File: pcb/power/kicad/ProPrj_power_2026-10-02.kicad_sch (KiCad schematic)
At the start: 0 parts

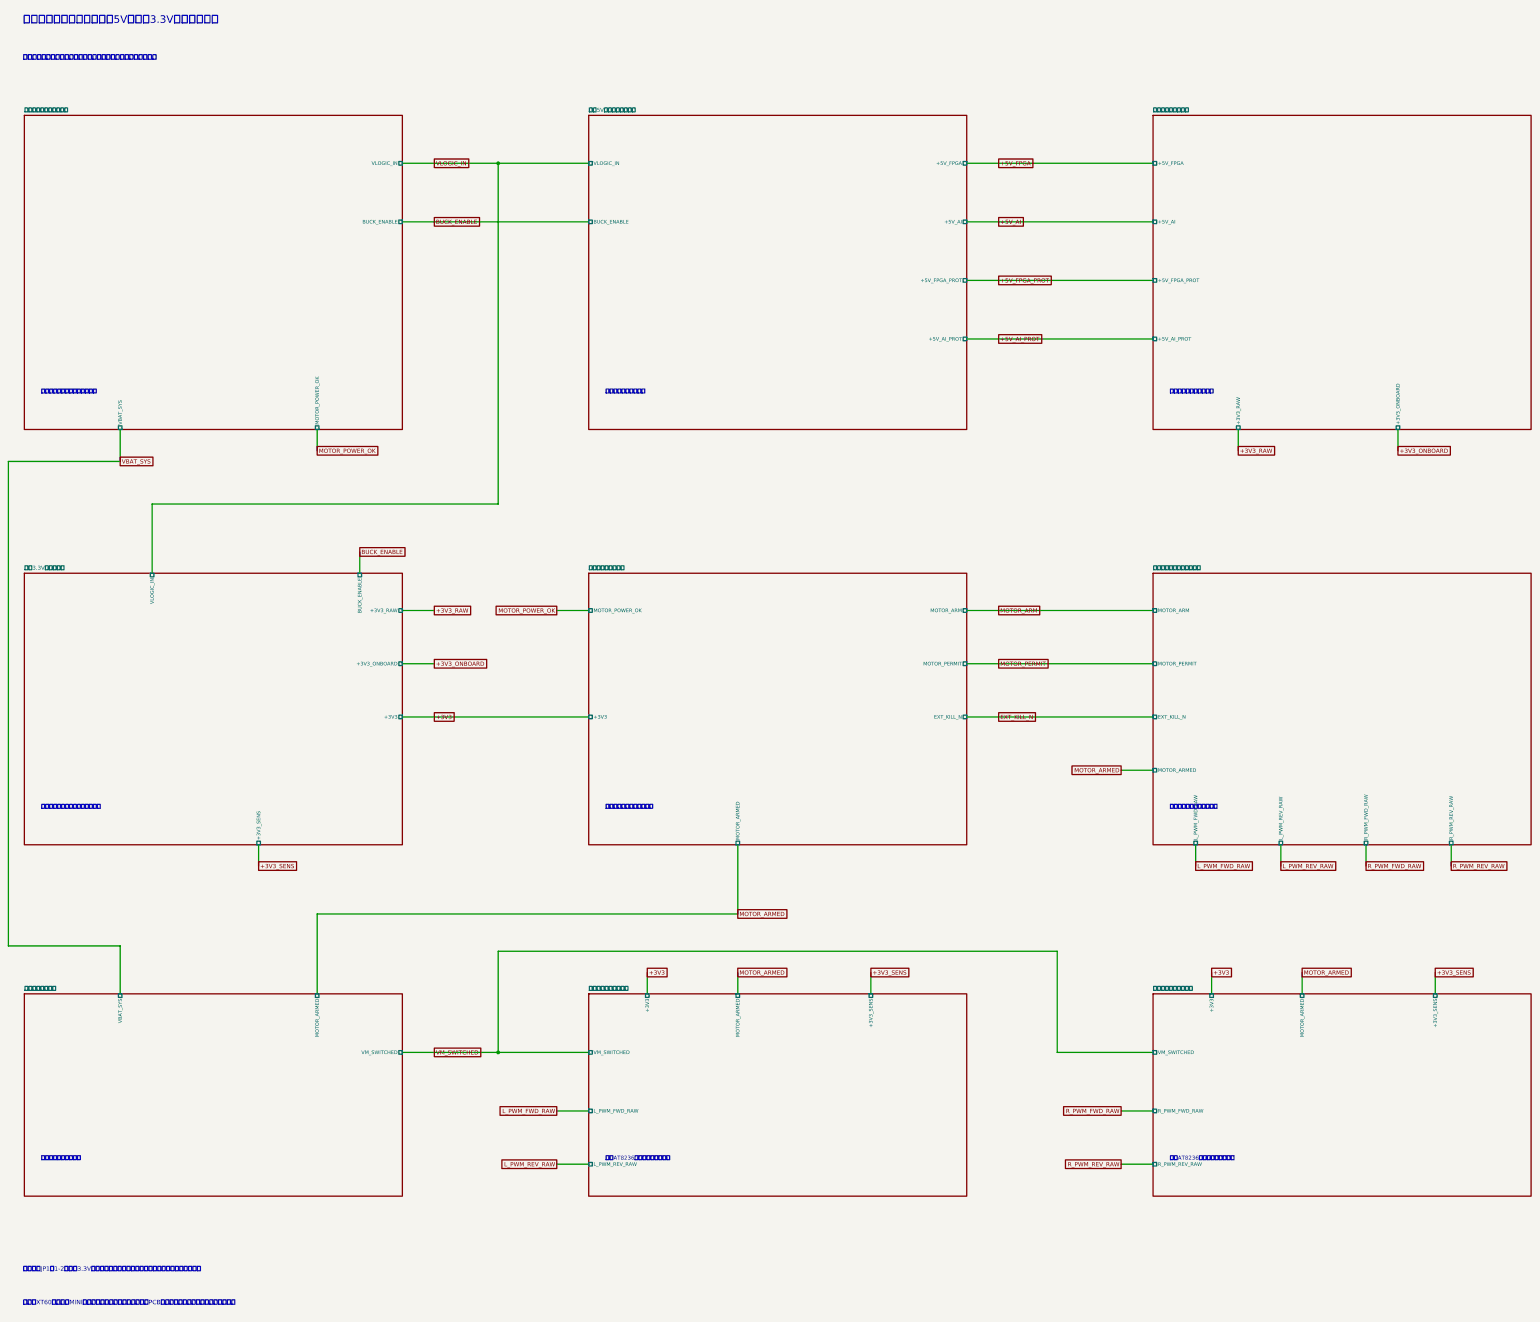
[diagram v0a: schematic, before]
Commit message: 10.4
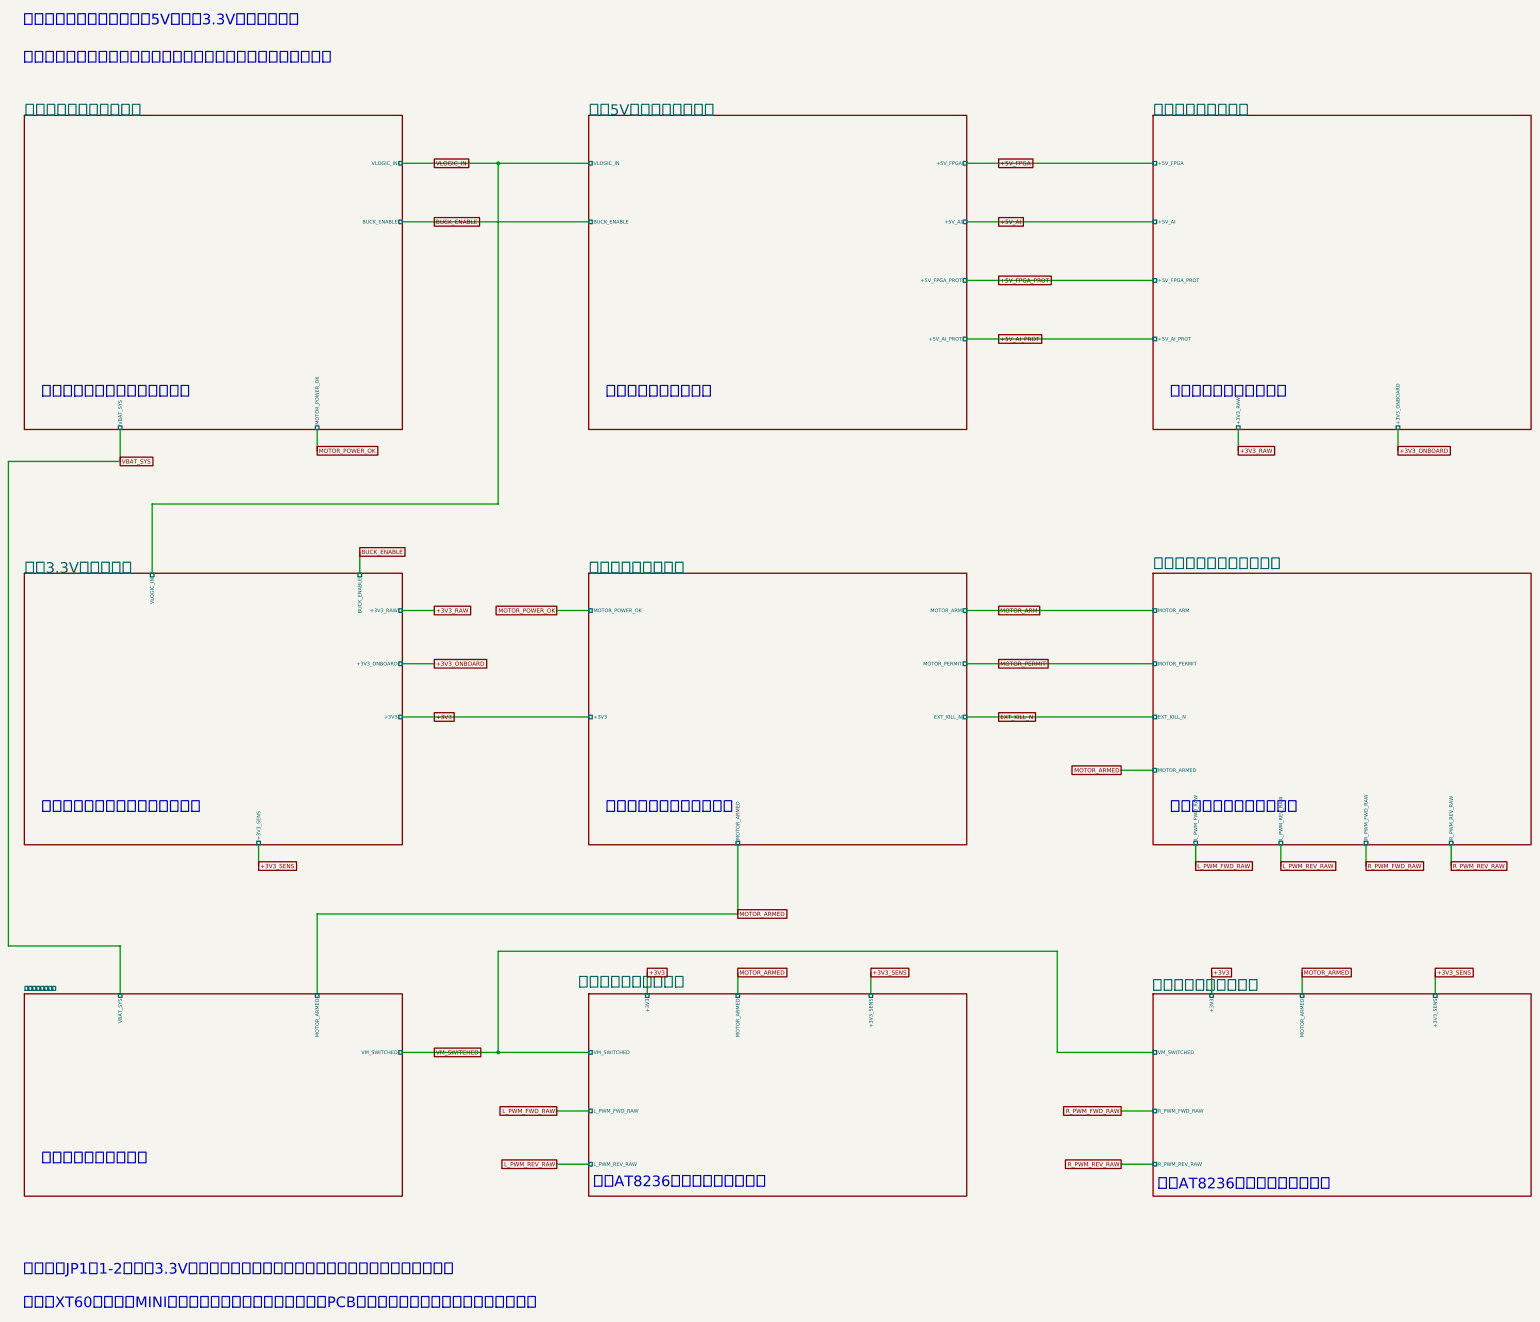
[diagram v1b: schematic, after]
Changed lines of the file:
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@@
 		(effects
 			(font
-				(size 0.95 0.95)
+				(size 2.54 2.54)
 			)
 			(justify left)
@@
 		(effects
 			(font
-				(size 1.05 1.05)
+				(size 2.54 2.54)
 			)
 			(justify left)
@@
 	(text "右侧AT8236、编码器与电流监测"
 		(exclude_from_sim no)
-		(at 293.56 289.56 0)
-		(effects
-			(font
-				(size 0.95 0.95)
+		(at 290.576 295.656 0)
+		(effects
+			(font
+				(size 2.54 2.54)
 			)
 			(justify left)
@@
 		(effects
 			(font
-				(size 0.95 0.95)
+				(size 2.54 2.54)
 			)
 			(justify left)
@@
 		(effects
 			(font
-				(size 0.95 0.95)
+				(size 2.54 2.54)
 			)
 			(justify left)
@@
 		(effects
 			(font
-				(size 0.95 0.95)
+				(size 2.54 2.54)
 			)
 			(justify left)
@@
 		(effects
 			(font
-				(size 1.1 1.1)
+				(size 2.54 2.54)
 			)
 			(justify left)
@@
 		(effects
 			(font
-				(size 0.95 0.95)
+				(size 2.54 2.54)
 			)
 			(justify left)
@@
 	(text "左侧AT8236、编码器与电流监测"
 		(exclude_from_sim no)
-		(at 158.94 289.56 0)
-		(effects
-			(font
-				(size 0.95 0.95)
+		(at 155.956 295.148 0)
+		(effects
+			(font
+				(size 2.54 2.54)
 			)
 			(justify left)
@@
 		(effects
 			(font
-				(size 0.95 0.95)
+				(size 2.54 2.54)
 			)
 			(justify left)
@@
 		(effects
 			(font
-				(size 0.95 0.95)
+				(size 2.54 2.54)
 			)
 			(justify left)
@@
 		(effects
 			(font
-				(size 1.05 1.05)
+				(size 2.54 2.54)
 			)
 			(justify left)
@@
 		(effects
 			(font
-				(size 1.8 1.8)
+				(size 2.54 2.54)
 			)
 			(justify left)
@@
 		)
 		(property "Sheetname" "右电机驱动与电流监测"
-			(at 289.56 248.92 0)
-			(show_name no)
-			(do_not_autoplace no)
-			(effects
-				(font
-					(size 0.95 0.95)
+			(at 289.306 248.158 0)
+			(show_name no)
+			(do_not_autoplace no)
+			(effects
+				(font
+					(size 2.54 2.54)
 				)
 				(justify left)
@@
 					(size 0.85 0.85)
 				)
+				(justify left)
 			)
 		)
@@
 					(size 0.85 0.85)
 				)
+				(justify right)
 			)
 		)
@@
 					(size 0.85 0.85)
 				)
+				(justify right)
 			)
 		)
@@
 					(size 0.85 0.85)
 				)
+				(justify right)
 			)
 		)
@@
 					(size 0.85 0.85)
 				)
+				(justify left)
 			)
 		)
@@
 					(size 0.85 0.85)
 				)
+				(justify left)
 			)
 		)
@@
 		)
 		(property "Sheetname" "左电机驱动与电流监测"
-			(at 154.94 248.92 0)
-			(show_name no)
-			(do_not_autoplace no)
-			(effects
-				(font
-					(size 0.95 0.95)
+			(at 152.4 247.396 0)
+			(show_name no)
+			(do_not_autoplace no)
+			(effects
+				(font
+					(size 2.54 2.54)
 				)
 				(justify left)
@@
 					(size 0.85 0.85)
 				)
+				(justify left)
 			)
 		)
@@
 					(size 0.85 0.85)
 				)
+				(justify right)
 			)
 		)
@@
 					(size 0.85 0.85)
 				)
+				(justify right)
 			)
 		)
@@
 					(size 0.85 0.85)
 				)
+				(justify right)
 			)
 		)
@@
 					(size 0.85 0.85)
 				)
+				(justify left)
 			)
 		)
@@
 					(size 0.85 0.85)
 				)
+				(justify left)
 			)
 		)
@@
 			(effects
 				(font
-					(size 0.95 0.95)
+					(size 2.54 2.54)
 				)
 				(justify left)
@@
 			(effects
 				(font
-					(size 0.95 0.95)
+					(size 2.54 2.54)
 				)
 				(justify left)
@@
 			(effects
 				(font
-					(size 0.95 0.95)
+					(size 2.54 2.54)
 				)
 				(justify left)
@@
 			(effects
 				(font
-					(size 0.95 0.95)
+					(size 2.54 2.54)
 				)
 				(justify left)
@@
 		)
 		(property "Sheetname" "逻辑板控制与电源监测接口"
-			(at 289.56 148.59 0)
-			(show_name no)
-			(do_not_autoplace no)
-			(effects
-				(font
-					(size 0.95 0.95)
+			(at 289.56 147.574 0)
+			(show_name no)
+			(do_not_autoplace no)
+			(effects
+				(font
+					(size 2.54 2.54)
 				)
 				(justify left)
@@
 			(effects
 				(font
-					(size 0.95 0.95)
+					(size 2.54 2.54)
 				)
 				(justify left)
